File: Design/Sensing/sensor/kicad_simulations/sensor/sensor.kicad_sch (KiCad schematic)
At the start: 44 parts, among them J1 Conn_02x14_Counter_Clockwise, J10 L_S_B, J11 Conn_01x01_Pin, J12 Conn_01x02_Pin, J13 Conn_01x02_Pin, J14 Conn_01x02_Pin, J15 Conn_01x02_Pin, J16 Conn_01x01_Pin, J17 Conn_01x02_Pin, J18 Conn_01x01_Pin, J3 Conn_01x02_Pin, J4 Conn_01x02_Pin, J5 Conn_01x02_Pin, J6 Conn_01x01_Pin, J7 Conn_01x02_Pin, J8 Conn_01x02_Pin, J9 Conn_01x02_Pin, Q1 MMBT2222A, Q2 MMBT2222A, Q3 MMBT2222A, U1 TSSP58038, U2 TSSP58038, U3 TSSP58038, U4 BUF602xD, U5 BUF602xD, U6 BUF602xD

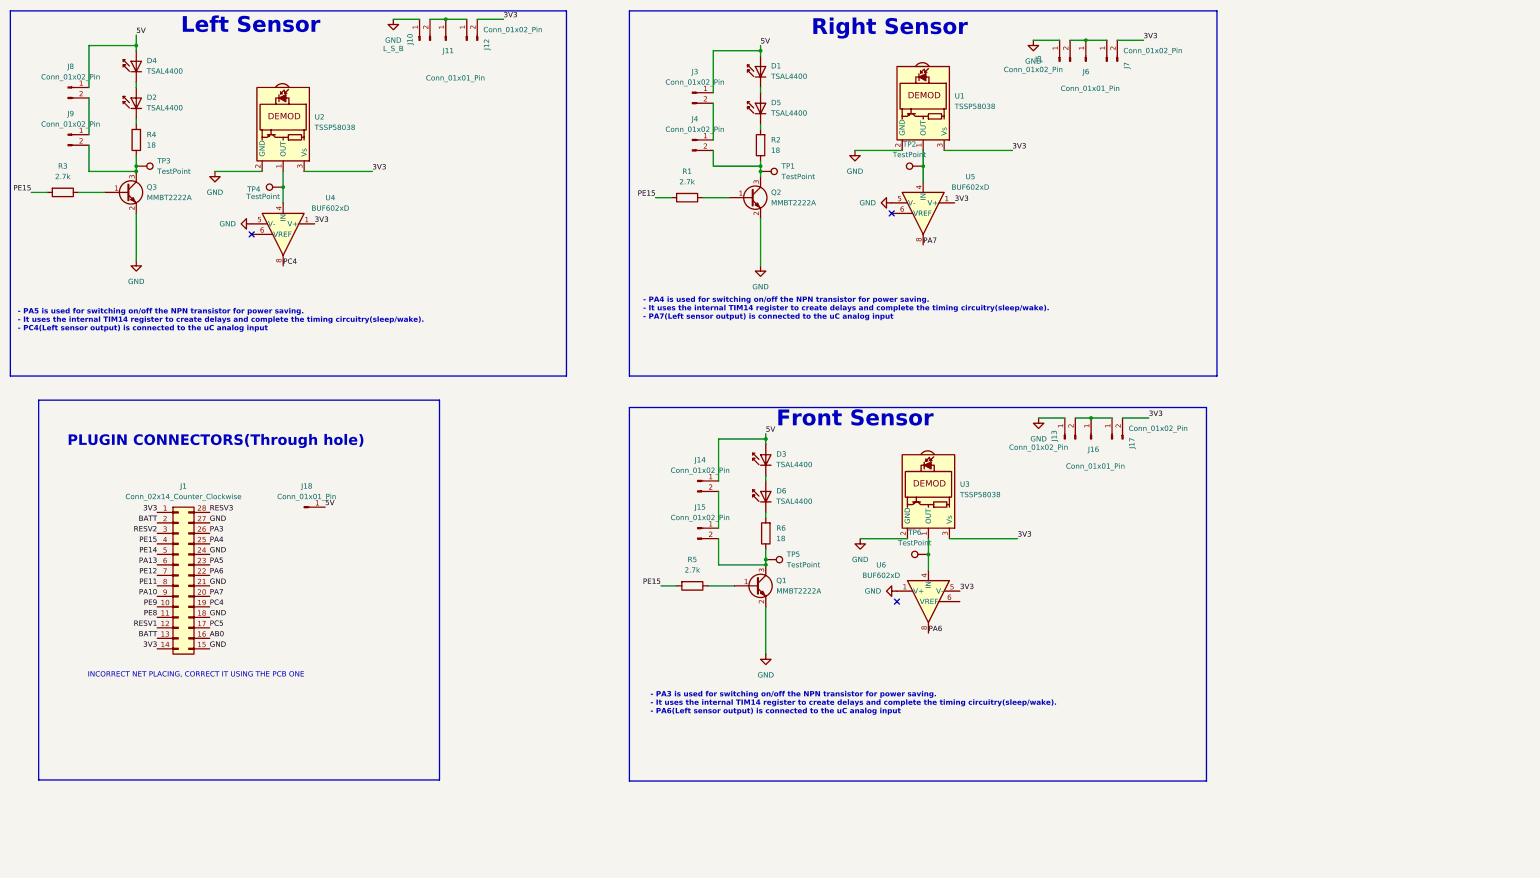
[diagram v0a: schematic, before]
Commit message: pcb placement redo
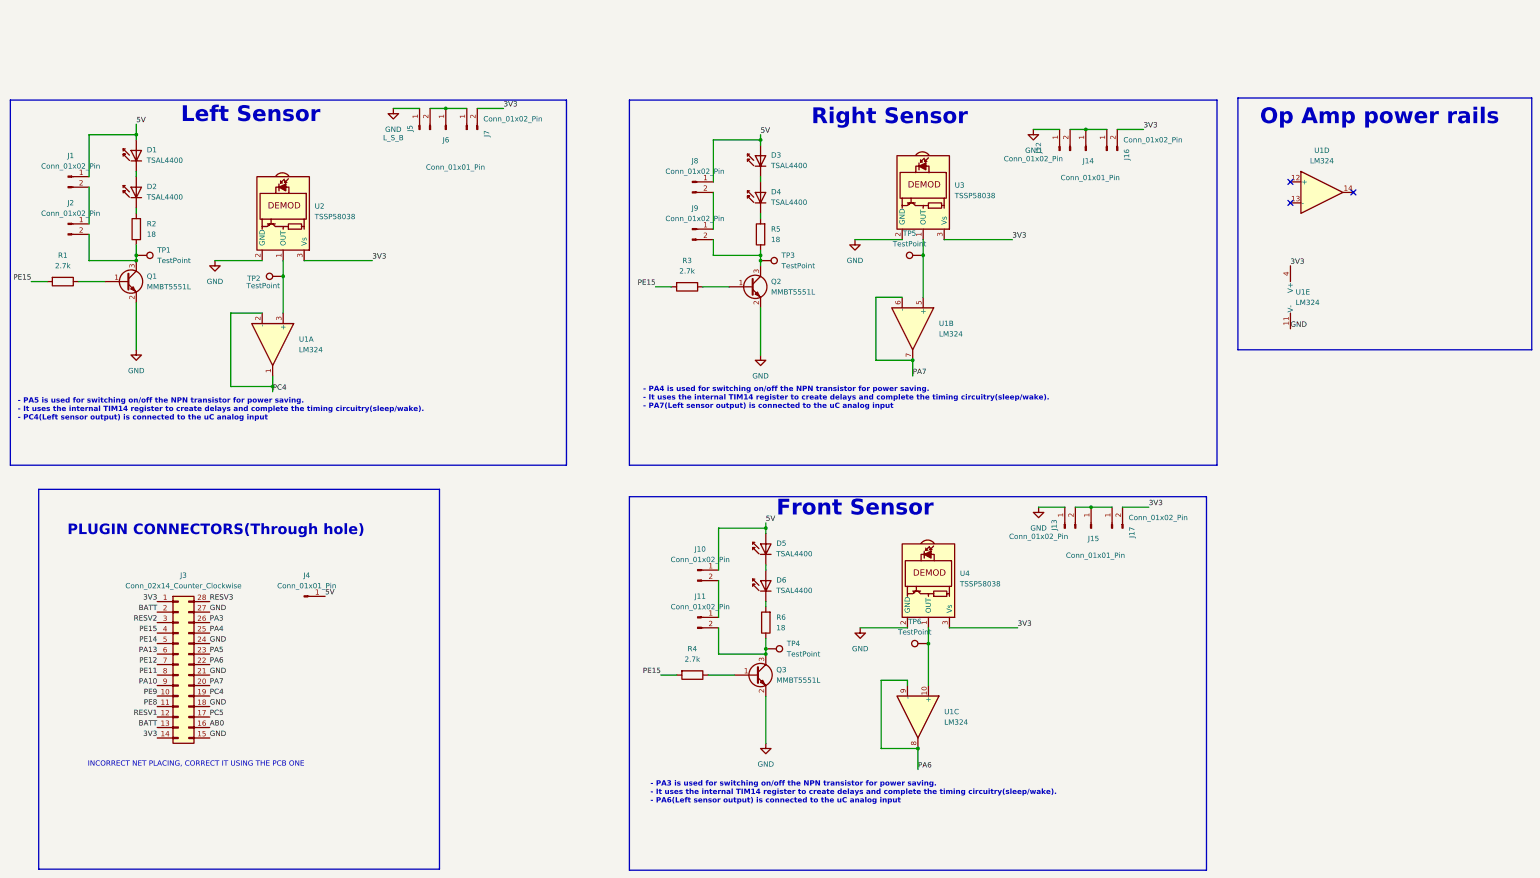
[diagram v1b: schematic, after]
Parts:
- removed J1: Conn_02x14_Counter_Clockwise, Connector_PinSocket_2.54mm:PinSocket_2x14_P2.54mm_Vertical, symbol Connector_Generic:Conn_02x14_Counter_Clockwise
- removed J11, J16, J18: Conn_01x01_Pin, Connector_PinHeader_2.54mm:PinHeader_1x01_P2.54mm_Vertical, symbol Connector:Conn_01x01_Pin
- removed J14, J15, J3, J4: Conn_01x02_Pin, Connector_PinHeader_2.54mm:PinHeader_1x02_P2.54mm_Vertical, symbol Connector:Conn_01x02_Pin
- removed Q1, Q2, Q3: MMBT2222A, Package_TO_SOT_SMD:SOT-23, symbol Transistor_BJT:MMBT2222A
- removed U1: TSSP58038, OptoDevice:Vishay_MINICAST-3Pin, symbol Sensor_Proximity:TSSP58038
- removed U4, U5, U6: BUF602xD, Package_SO:SOIC-8_3.9x4.9mm_P1.27mm, symbol Amplifier_Buffer:BUF602xD
- added J1, J11, J16, J2: Conn_01x02_Pin, Connector_PinHeader_2.54mm:PinHeader_1x02_P2.54mm_Vertical, symbol Connector:Conn_01x02_Pin
- added J14, J15, J4: Conn_01x01_Pin, Connector_PinHeader_2.54mm:PinHeader_1x01_P2.54mm_Vertical, symbol Connector:Conn_01x01_Pin
- added J3: Conn_02x14_Counter_Clockwise, Connector_PinSocket_2.54mm:PinSocket_2x14_P2.54mm_Vertical, symbol Connector_Generic:Conn_02x14_Counter_Clockwise
- added Q1, Q2, Q3: MMBT5551L, Package_TO_SOT_SMD:SOT-23, symbol Transistor_BJT:MMBT5551L
- added U1: LM324, Package_SO:SOIC-14_3.9x8.7mm_P1.27mm, symbol Amplifier_Operational:LM324
- added U4: TSSP58038, OptoDevice:Vishay_MINICAST-3Pin, symbol Sensor_Proximity:TSSP58038
- J10: value L_S_B -> Conn_01x02_Pin
- J5: value Conn_01x02_Pin -> L_S_B
- R4: value 18 -> 2.7k
- R5: value 2.7k -> 18
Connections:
- net 3V3: now also J16.2 (Pin_2), J3.1 (Pin_1), J3.14 (Pin_14), U1.4 (V+), U4.3 (Vs); no longer J12.2 (Pin_2)
- net 5V: now also D5.2 (A), J10.1 (Pin_1), J1.1 (Pin_1), J4.1 (Pin_1); no longer D4.2 (A)
- net AB0: now also J3.16 (Pin_16)
- net BATT: now also J3.13 (Pin_13), J3.2 (Pin_2)
- net GND: now also J12.1 (Pin_1), J3.15 (Pin_15), J3.18 (Pin_18), J3.21 (Pin_21), J3.24 (Pin_24), J3.27 (Pin_27), Q1.2 (E), Q2.2 (E), Q3.2 (E), U1.11 (V-), U4.2 (GND); no longer J10.1 (Pin_1)
- net PA10: now also J3.9 (Pin_9)
- net PA13: now also J3.6 (Pin_6)
- net PA3: now also J3.26 (Pin_26)
- net PA4: now also J3.25 (Pin_25)
- net PA5: now also J3.23 (Pin_23)
- net PA6: now also J3.22 (Pin_22), U1.8, U1.9 (-)
- net PA7: now also J3.20 (Pin_20), U1.6 (-), U1.7
- net PC4: now also J3.19 (Pin_19), U1.1, U1.2 (-)
- net PC5: now also J3.17 (Pin_17)
- net PE11: now also J3.8 (Pin_8)
- net PE12: now also J3.7 (Pin_7)
- net PE14: now also J3.5 (Pin_5)
- net PE15: now also R4.2, J3.4 (Pin_4); no longer R5.2
- net PE8: now also J3.11 (Pin_11)
- net PE9: now also J3.10 (Pin_10)
- net RESV1: now also J3.12 (Pin_12)
- net RESV2: now also J3.3 (Pin_3)
- net RESV3: now also J3.28 (Pin_28)
- net at J10.2 (Pin_2): now also J11.1 (Pin_1); no longer J12.1 (Pin_1)
- net at D4.1 (K): now also R5.2; no longer D2.2 (A)
- net at U3.1 (OUT): now also TP5.1, U1.5 (+); no longer TP6.1
- net at TP4.1: now also R6.1, J11.2 (Pin_2), Q3.3 (C); no longer U2.1 (OUT)
- net at D2.1 (K): now also R2.2; no longer R4.2
- net at J9.2 (Pin_2), TP3.1: now also R5.1, Q2.3 (C); no longer R4.1
- net at D3.1 (K): now also D4.2 (A); no longer D6.2 (A)
- net at D5.1 (K): now also D6.2 (A); no longer R2.2
- net at D1.1 (K): now also D2.2 (A); no longer D5.2 (A)
- net at R3.1: now also Q2.1 (B)
- net at J13.2 (Pin_2), J17.1 (Pin_1): now also J15.1 (Pin_1)
- net at R1.1: now also Q1.1 (B)
- net at TP2.1: now also U2.1 (OUT), U1.3 (+)
- net at R2.1, TP1.1: now also J2.2 (Pin_2), Q1.3 (C)
- new net: J12.2 (Pin_2), J14.1 (Pin_1), J16.1 (Pin_1)
- new net: Q3.1 (B), R4.1
- new net: TP6.1, U1.10 (+), U4.1 (OUT)
- new net: J1.2 (Pin_2), J2.1 (Pin_1)
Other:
- note added: "Op Amp power rails"
